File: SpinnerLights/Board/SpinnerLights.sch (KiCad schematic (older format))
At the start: 4 parts

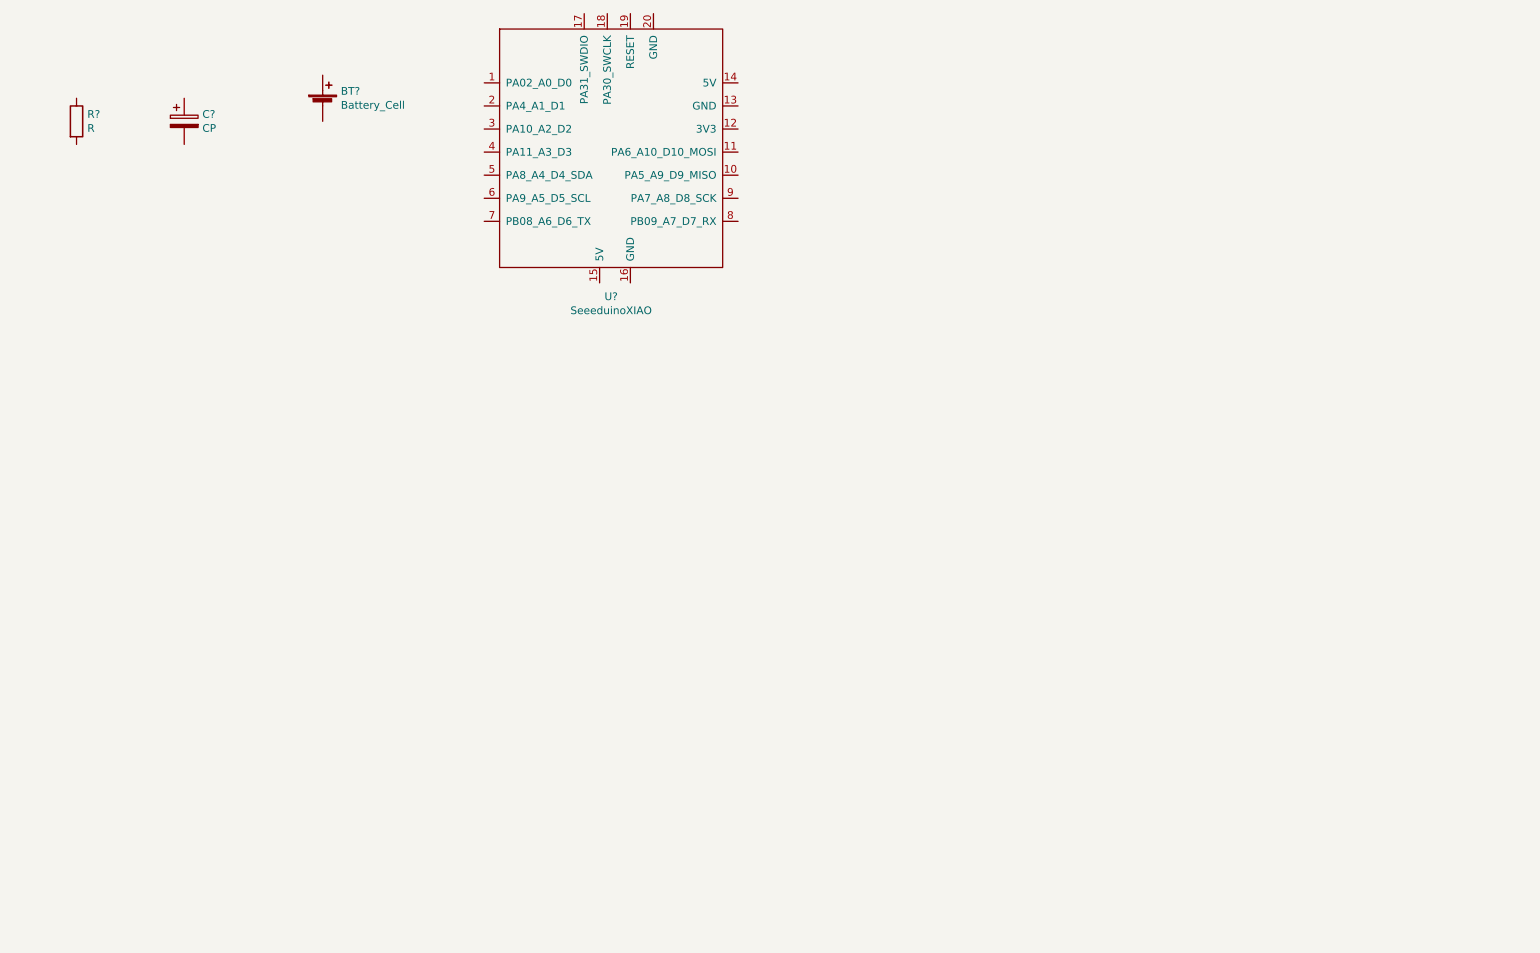
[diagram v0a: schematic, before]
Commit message: WIP on SpinnerLights board
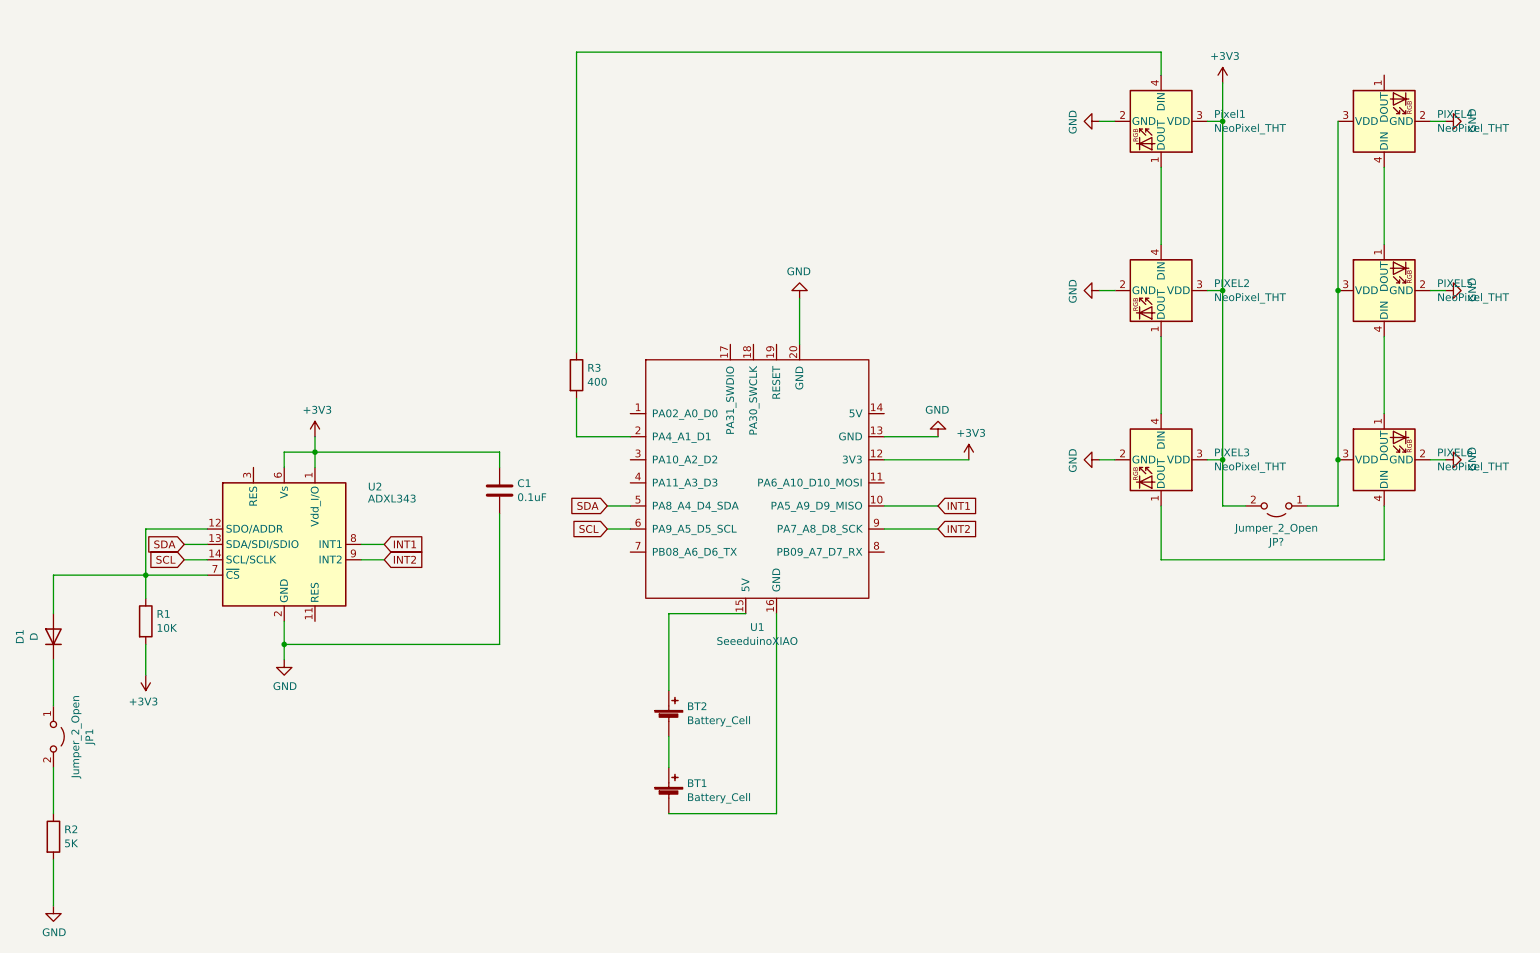
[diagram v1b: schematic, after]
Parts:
- removed C?: CP, symbol Device:CP
- removed R?: R, symbol Device:R
- added BT1: Battery_Cell, symbol Device:Battery_Cell
- added C1: 0.1uF, symbol Device:C
- added D1: D, symbol Device:D
- added JP1, JP?: Jumper_2_Open, symbol Jumper:Jumper_2_Open
- added PIXEL2, PIXEL3, PIXEL4, PIXEL5, PIXEL6, Pixel1: NeoPixel_THT, symbol LED:NeoPixel_THT
- added R1: 10K, symbol Device:R
- added R2: 5K, symbol Device:R
- added R3: 400, symbol Device:R
- added U2: ADXL343, Package_LGA:LGA-14_3x5mm_P0.8mm_LayoutBorder1x6y, symbol Sensor_Motion:ADXL343
- gave numbers to parts that had none: 2
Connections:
- net at BT2.1 (+): now also U1.15 (5V)
- net at BT2.2 (-): now also BT1.1 (+)
- net INT1: now reaches U1.10 (PA5_A9_D9_MISO)
- net INT1: now also U2.8 (INT1)
- net +3V3: now reaches U1.12 (3V3)
- net +3V3: now also C1.1, JP?.2 (B), PIXEL2.3 (VDD), PIXEL3.3 (VDD), Pixel1.3 (VDD), R1.2, U2.1 (Vdd_I/O), U2.6 (Vs)
- net GND: now reaches U1.13 (GND)
- net GND: now also U1.20 (GND), C1.2, PIXEL2.2 (GND), PIXEL3.2 (GND), PIXEL4.2 (GND), PIXEL5.2 (GND), PIXEL6.2 (GND), Pixel1.2 (GND), R2.2, U2.2 (GND), U2.4 (GND), U2.5 (GND)
- net at U1.16 (GND): now also BT1.2 (-)
- net at U1.2 (PA4_A1_D1): now also R3.2
- net SDA: now reaches U1.5 (PA8_A4_D4_SDA)
- net SDA: now also U2.13 (SDA/SDI/SDIO)
- net SCL: now reaches U1.6 (PA9_A5_D5_SCL)
- net SCL: now also U2.14 (SCL/SCLK)
- net INT2: now reaches U1.9 (PA7_A8_D8_SCK)
- net INT2: now also U2.9 (INT2)
- new net: D1.1 (K), JP1.1 (A)
- new net: D1.2 (A), R1.1, U2.12 (SDO/ADDR), U2.7 (~CS)
- new net: JP1.2 (B), R2.1
- new net: PIXEL2.4 (DIN), Pixel1.1 (DOUT)
- new net: Pixel1.4 (DIN), R3.1
- new net: PIXEL2.1 (DOUT), PIXEL3.4 (DIN)
- new net: PIXEL3.1 (DOUT), PIXEL6.4 (DIN)
- new net: PIXEL5.4 (DIN), PIXEL6.1 (DOUT)
- new net: JP?.1 (A), PIXEL4.3 (VDD), PIXEL5.3 (VDD), PIXEL6.3 (VDD)
- new net: PIXEL4.4 (DIN), PIXEL5.1 (DOUT)
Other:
- moved on the sheet: BT2, U1
